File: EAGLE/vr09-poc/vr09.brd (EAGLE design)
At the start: 80 x 60 mm, 24 parts, among them K00 MX-5-PIN-HOTSWAP, K01 MX-5-PIN-HOTSWAP, K02 MX-5-PIN-HOTSWAP, K10 MX-5-PIN-HOTSWAP, K11 MX-5-PIN-HOTSWAP, K12 MX-5-PIN-HOTSWAP

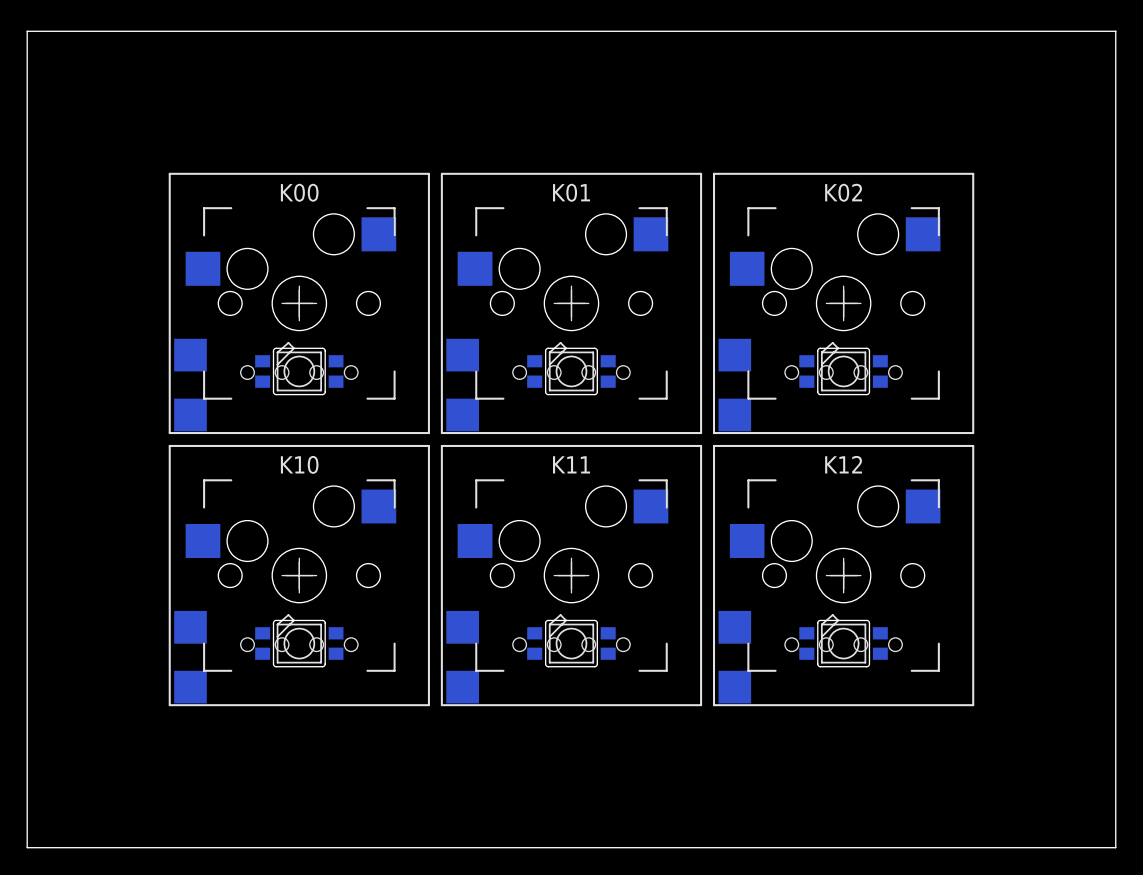
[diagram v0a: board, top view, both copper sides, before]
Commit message: wip
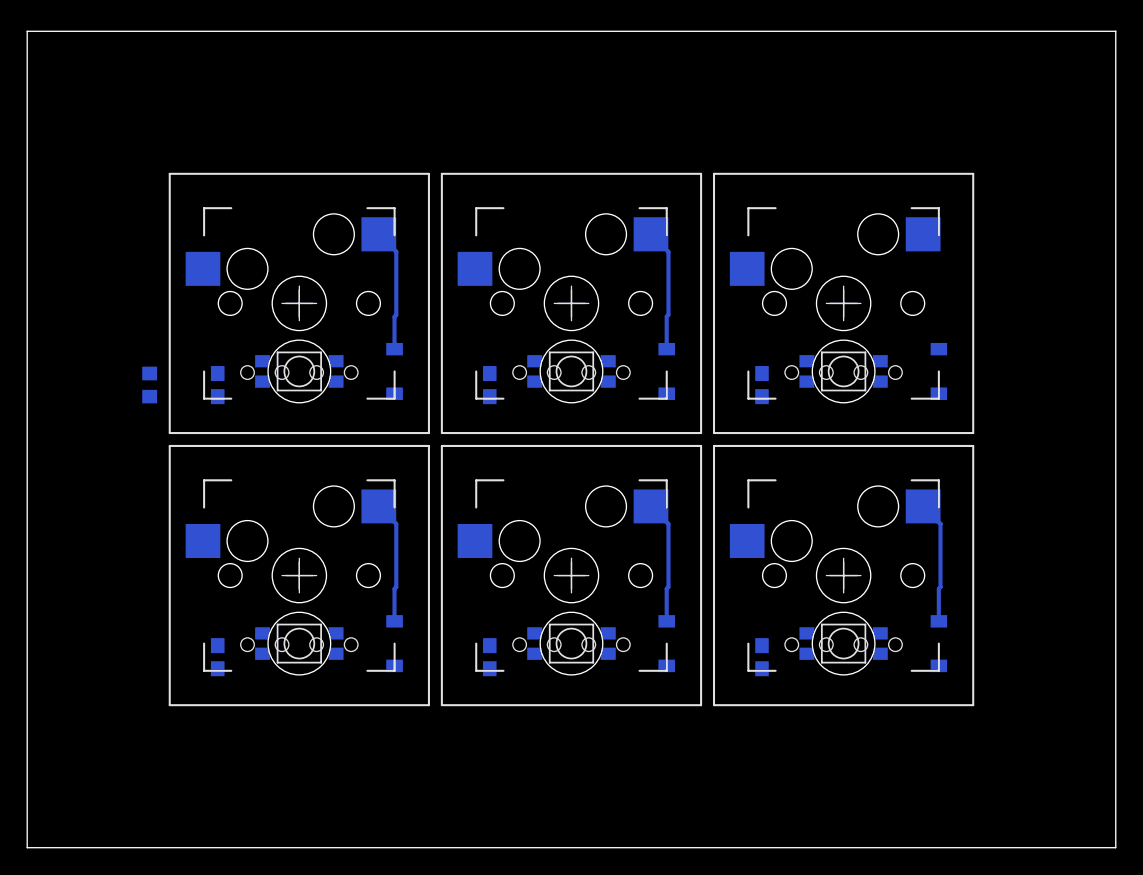
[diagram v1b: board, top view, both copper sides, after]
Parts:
- removed D1, D2, D3, D4, D5, D6: (no value), diode:SMB
- removed U$10, U$11, U$12, U$7, U$8, U$9: SK6812-E-REVERSE, ts_keyboards:SK6812-E
- added C00, C01, C02, C10, C11, C12: 100nF, rcl:C0603
- added D00, D01, D02, D10, D11, D12: (no value), jlcpcb_basic_parts:SOD-123
- added L00, L01, L02, L10, L11, L12: SK6812-E-REVERSEDRILL, ts_keyboards:SK6812-E-DRILL
- added R1: 500ohm, rcl:R0603
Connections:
- removed net N$10: U$10.4-DIN, U$9.2-DOUT
- removed net N$8: D6.A, K12.P$1
- removed net N$9: U$8.2-DOUT, U$9.4-DIN
- new net DIN: R1.1
- new net N$13: L11.2-DOUT, L12.4-DIN
- new net N$14: L10.2-DOUT, L11.4-DIN
- new net N$19: L02.2-DOUT, L10.4-DIN
- net COL1: now also K00.P$1, K10.P$1; no longer D1.C, D4.C
- net COL2: now also K01.P$1, K11.P$1; no longer D2.C, D5.C
- net COL3: now also K02.P$1, K12.P$1; no longer D3.C, D6.C
- net GND: now also C00.2, C01.2, C02.2, C10.2, C11.2, C12.2, L00.3-GND, L01.3-GND, L02.3-GND, L10.3-GND, L11.3-GND, L12.3-GND; no longer U$10.3-GND, U$11.3-GND, U$12.3-GND, U$7.3-GND, U$8.3-GND, U$9.3-GND
- net N$1: now also D10.A, K10.P$2; no longer U$7.4-DIN
- net N$11: now also L00.2-DOUT, L01.4-DIN; no longer U$10.2-DOUT, U$11.4-DIN
- net N$12: now also L01.2-DOUT, L02.4-DIN; no longer U$11.2-DOUT, U$12.4-DIN
- net N$2: now also D11.A, K11.P$2; no longer D4.A, K10.P$1
- net N$3: now also D12.A, K12.P$2; no longer D2.A, K01.P$1
- net N$4: now also D02.A, K02.P$2; no longer D1.A, K00.P$1
- net N$5: now also D01.A, K01.P$2; no longer D3.A, K02.P$1
- net N$6: now also L00.4-DIN, R1.2; no longer U$7.2-DOUT, U$8.4-DIN
- net N$7: now also D00.A, K00.P$2; no longer D5.A, K11.P$1
- net ROW1: now also D00.C, D01.C, D02.C; no longer K00.P$2, K01.P$2, K02.P$2
- net ROW2: now also D10.C, D11.C, D12.C; no longer K10.P$2, K11.P$2, K12.P$2
- net VCC: now also C00.1, C01.1, C02.1, C10.1, C11.1, C12.1, L00.1-VDD, L01.1-VDD, L02.1-VDD, L10.1-VDD, L11.1-VDD, L12.1-VDD; no longer U$10.1-VDD, U$11.1-VDD, U$12.1-VDD, U$7.1-VDD, U$8.1-VDD, U$9.1-VDD
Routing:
- net N$3: track 0.00 -> 9.02 mm
- net N$7: track 0.00 -> 9.02 mm
- net N$1: track 0.00 -> 9.02 mm
- net N$5: track 0.00 -> 9.02 mm
- net N$2: track 0.00 -> 9.02 mm

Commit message: wip
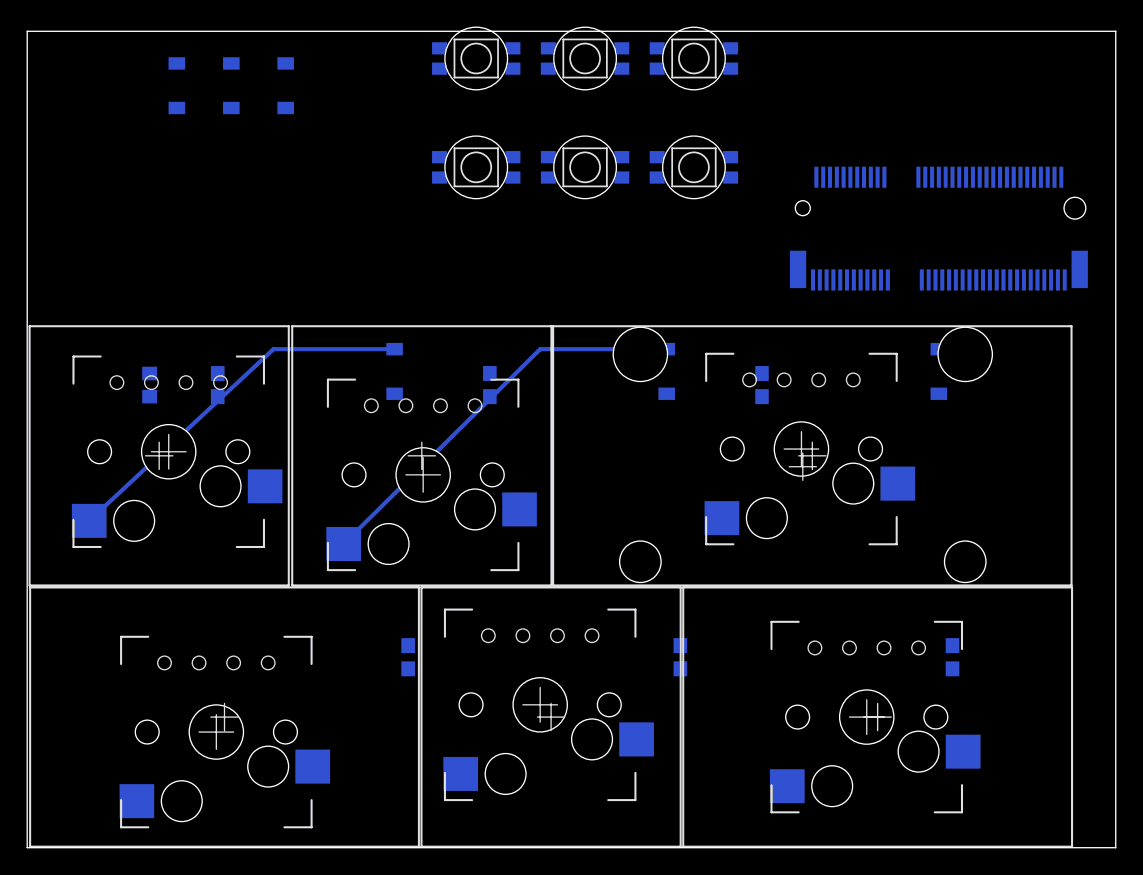
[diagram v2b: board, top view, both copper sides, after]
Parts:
- added J1: MICROMOD-2222-C, SparkFun-MicroMod:M.2-CONNECTOR-E
- added U$7: (no value), ts_keyboards:MX-STABS-200U
- U$3: value MX-FPRINT-1905-100U -> MX-FPRINT-1905-200U; device ts_keyboards:MX-FPRINT-1905-100U -> ts_keyboards:MX-FPRINT-1905-200U
- U$4, U$6: value MX-FPRINT-1905-100U -> MX-FPRINT-1905-150U; device ts_keyboards:MX-FPRINT-1905-100U -> ts_keyboards:MX-FPRINT-1905-150U
- moved D12 63.1 mm to (19.0, 56.0)
- moved D11 52.0 mm to (15.0, 56.0)
- moved D10 44.0 mm to (11.0, 56.0)
- moved L10 37.3 mm to (33.0, 50.0)
- moved L12 36.7 mm to (49.0, 50.0)
- moved L11 35.0 mm to (41.0, 50.0)
- moved L00 26.4 mm to (33.0, 58.0)
- moved L02 25.5 mm to (49.0, 58.0)
- moved L01 23.0 mm to (41.0, 58.0)
- moved K01 16.7 mm to (29.1, 27.4), turned to 180 degrees
- moved U$2 15.7 mm to (29.0, 28.8)
- moved U$1 15.2 mm to (9.70, 28.8)
- moved K00 14.5 mm to (10.4, 29.1), turned to 180 degrees
- moved C10 14.0 mm to (28.0, 14.0)
- moved C11 14.0 mm to (48.0, 14.0)
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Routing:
- net N$5: track 9.02 -> 29.6 mm
- net N$7: track 9.02 -> 27.4 mm
- net N$3: track 9.02 -> 0.00 mm
- net N$1: track 9.02 -> 0.00 mm
- net N$2: track 9.02 -> 0.00 mm
